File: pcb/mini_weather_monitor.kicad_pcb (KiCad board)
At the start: 2 copper layers, 135 x 72 mm, 22 parts, among them U2 4.0inch_SPI_MSP4021, U2_BME280 module_bme280, U3_BH1750 module_bh1750

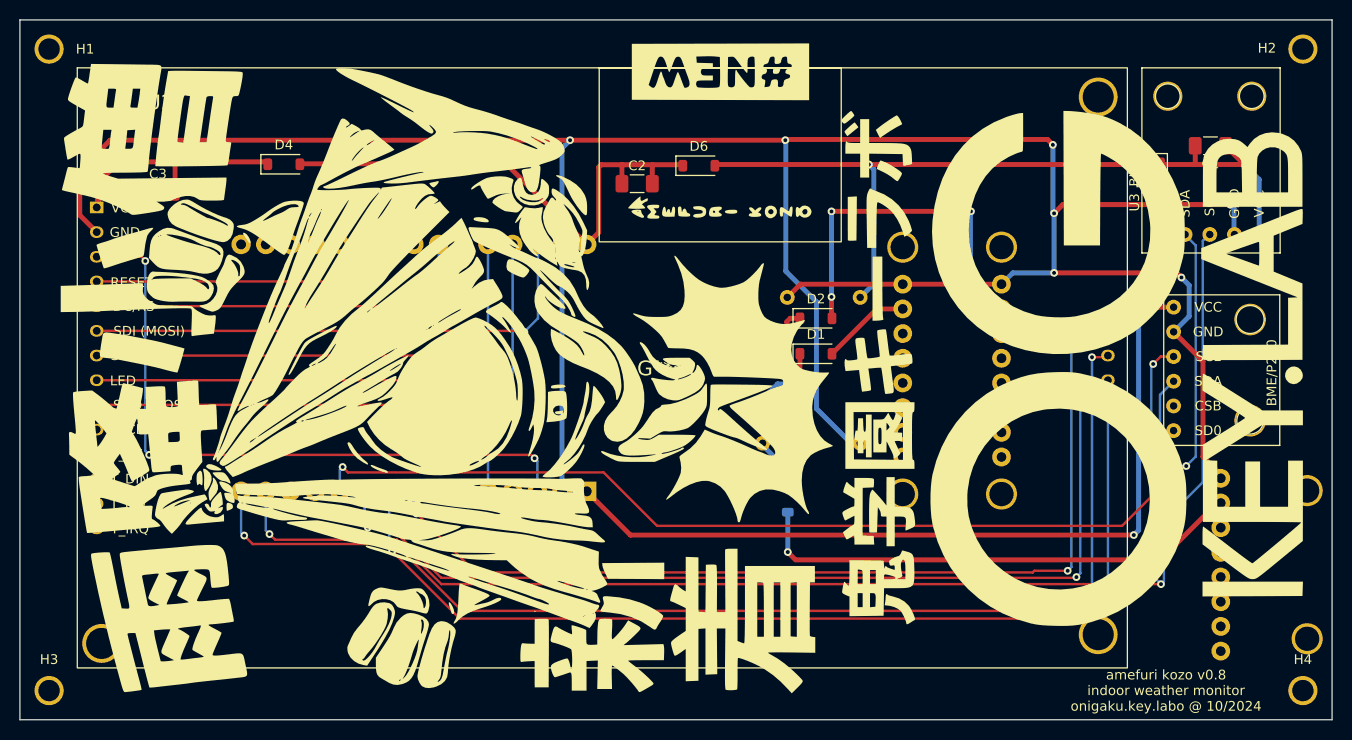
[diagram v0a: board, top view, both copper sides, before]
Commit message: working code. pcb wip
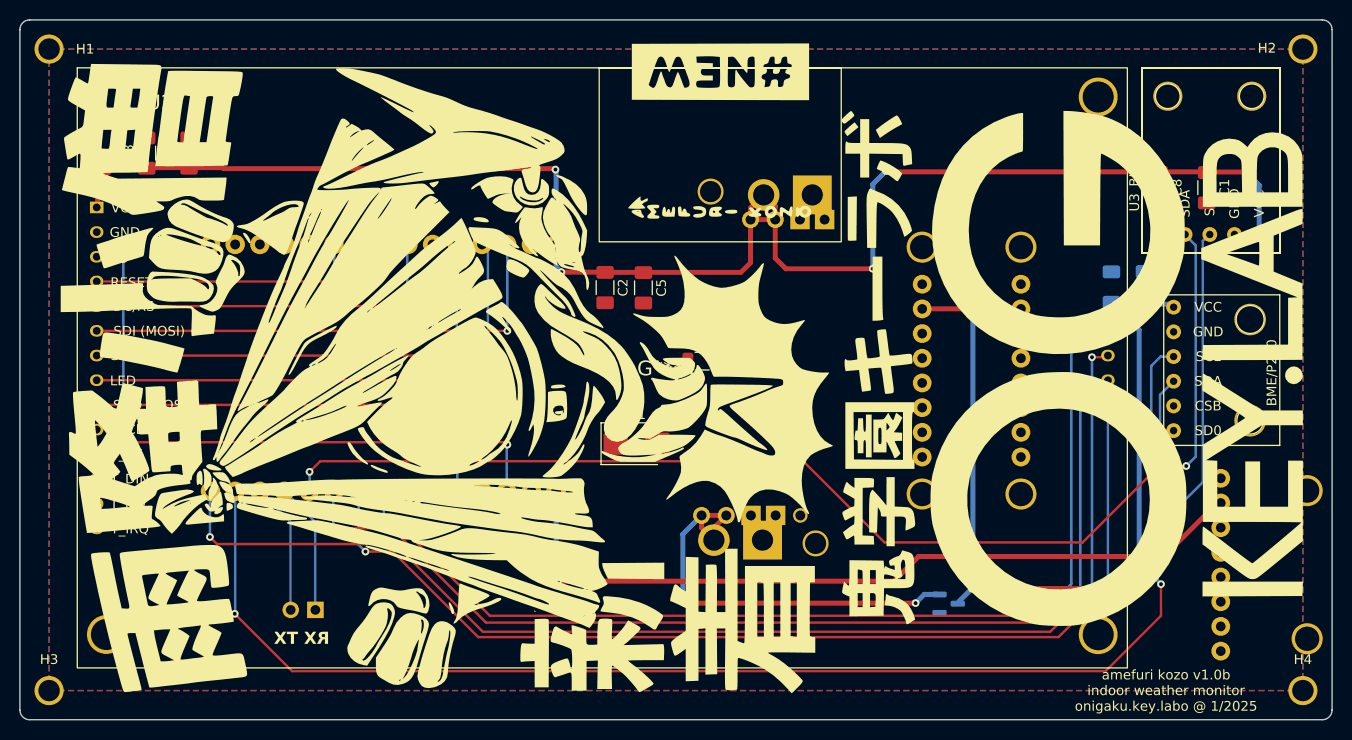
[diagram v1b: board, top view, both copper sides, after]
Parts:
- removed 5V_buck_boost1: ~, regulator_voltage:S09_HVN
- removed D2, D3, D4, D5, D6: 1N5819, Diode_SMD:D_SOD-123
- added C4: 100nF, Capacitor_SMD:C_1206_3216Metric_Pad1.33x1.80mm_HandSolder, B.Cu at (178.3, 91.5)
- added C5: 10uF, Capacitor_SMD:C_1206_3216Metric_Pad1.33x1.80mm_HandSolder, F.Cu at (130.2, 91.6)
- added C6: 10uF, Capacitor_SMD:C_1206_3216Metric_Pad1.33x1.80mm_HandSolder, F.Cu at (83.4, 77.7)
- added C7: 10uF, Capacitor_SMD:C_1206_3216Metric_Pad1.33x1.80mm_HandSolder, B.Cu at (181.7, 91.5)
- added C8: 10uF, Capacitor_SMD:C_1206_3216Metric_Pad1.33x1.80mm_HandSolder, F.Cu at (183.2, 81.2)
- added J1: Conn_01x02, Connector_PinHeader_2.54mm:PinHeader_1x02_P2.54mm_Vertical, B.Cu at (96.4, 124.7)
- added Q1: IRLML6402, Package_TO_SOT_SMD:SOT-23, B.Cu at (161.6, 124.1)
- added R2: 1k, Resistor_SMD:R_1206_3216Metric, F.Cu at (136.2, 99.1)
- added U1: ~, boost_converter:Pololu U3V70F5, B.Cu at (134.9, 120.1)
- C1, C2, C3: value C_Small -> 100nF
- D1: footprint Diode_SMD:D_SOD-123 -> Diode_SMD:D_SMB
- moved D1 20.6 mm to (129.4, 107.6)
- moved C2 11.2 mm to (126.2, 91.5), turned to -90 degrees
- moved C1 4.33 mm to (188.1, 81.3), turned to -90 degrees
- moved C3 4.16 mm to (79.0, 77.7), turned to 90 degrees
- moved U_ESP32_DEVKIT_V1 3.15 mm to (105.7, 99.8)
- moved adafruit_type_c_vertical_breakout1 2.00 mm to (164.0, 100.1)
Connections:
- C1 pad 1: Net-(D5-K) -> VCC
- C1 pad 2: Net-(D5-K) -> GND
- C2 pad 2: VCC -> GND
- C3 pad 1: Net-(D4-K) -> VCC
- C3 pad 2: Net-(D4-K) -> GND
- D1 pad 1: Net-(5V_buck_boost1-EN) -> VBUS
- U2 pad 1: Net-(D4-K) -> VCC
- U3_BH1750 pad 5: Net-(D5-K) -> VCC
- U_ESP32_DEVKIT_V1 pad 12: unconnected-(U_ESP32_DEVKIT_V1-RX0-Pad12) -> Net-(J1-Pin_1)
- U_ESP32_DEVKIT_V1 pad 13: unconnected-(U_ESP32_DEVKIT_V1-TX0-Pad13) -> Net-(J1-Pin_2)
- adafruit_type_c_breakout_rev_b1 pad 2: Net-(D3-A) -> Net-(Q1-D)
- adafruit_type_c_vertical_breakout1 pad 10: Net-(D2-A) -> Net-(Q1-D)
- adafruit_type_c_vertical_breakout1 pad 2: Net-(D1-A) -> Net-(Q1-D)
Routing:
- net GND: track 280.7 -> 0.69 mm, vias 7 -> 0
- net Net-(Q1-D): track 0.00 -> 71.4 mm, vias 0 -> 2
- net Net-(D3-A): track 52.2 -> 0.00 mm, vias 1 -> 0
- net VCC: track 111.9 -> 163.7 mm, vias 1 -> 5
- net VBUS: track 0.00 -> 44.9 mm, vias 0 -> 2
- net Net-(D2-A): track 38.6 -> 0.00 mm, vias 4 -> 0
- net Net-(5V_buck_boost1-EN): track 32.4 -> 0.00 mm, vias 1 -> 0
- net Net-(D4-K): track 29.3 -> 0.00 mm
- net Net-(D5-K): track 21.6 -> 0.00 mm, vias 1 -> 0
- net +3V3: track 84.8 -> 103.3 mm
- net Net-(U2_BME280-SCL): track 162.0 -> 179.9 mm, vias 3 -> 2
- net Net-(J1-Pin_1): track 0.00 -> 13.5 mm
- net Net-(J1-Pin_2): track 0.00 -> 13.5 mm
- net Net-(D1-A): track 9.19 -> 0.00 mm
- net Net-(U2-SD_CS): track 99.6 -> 108.0 mm
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- added copper zone on B.Cu, net GND
- added copper zone on F.Cu, net GND
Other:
- outline, holes or cut-outs redrawn
- board text added: "RX TX"
- board text added: "amefuri kozo v1.0b indoor weather monitor onigaku.key.labo @ 1/2025"
- board text removed: "amefuri kozo v0.8 indoor weather monitor onigaku.key.labo @ 10/2024"
